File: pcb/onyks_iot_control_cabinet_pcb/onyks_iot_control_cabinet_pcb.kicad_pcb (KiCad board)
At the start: 2 copper layers, 80 x 90 mm, 41 parts, among them J1 Conn_01x02_Socket, J10 Conn_02x05_Odd_Even, J2 Conn_01x06_Socket, J3 Screw_Terminal_01x02, J4 Jack-DC, J5 Conn_01x03_Pin, J6 Conn_02x09_Odd_Even, J7 Screw_Terminal_01x02, J8 Conn_01x06_Pin, Q1 SQ4050EY-T1_GE3, Q2 SQ4050EY-T1_GE3, Q3 NPN, Q4 NPN, SW1 SW_Push, SW2 SW_Push, SW3 SW_Push, U1 ESP32-WROOM-32D, U2 LMR51430

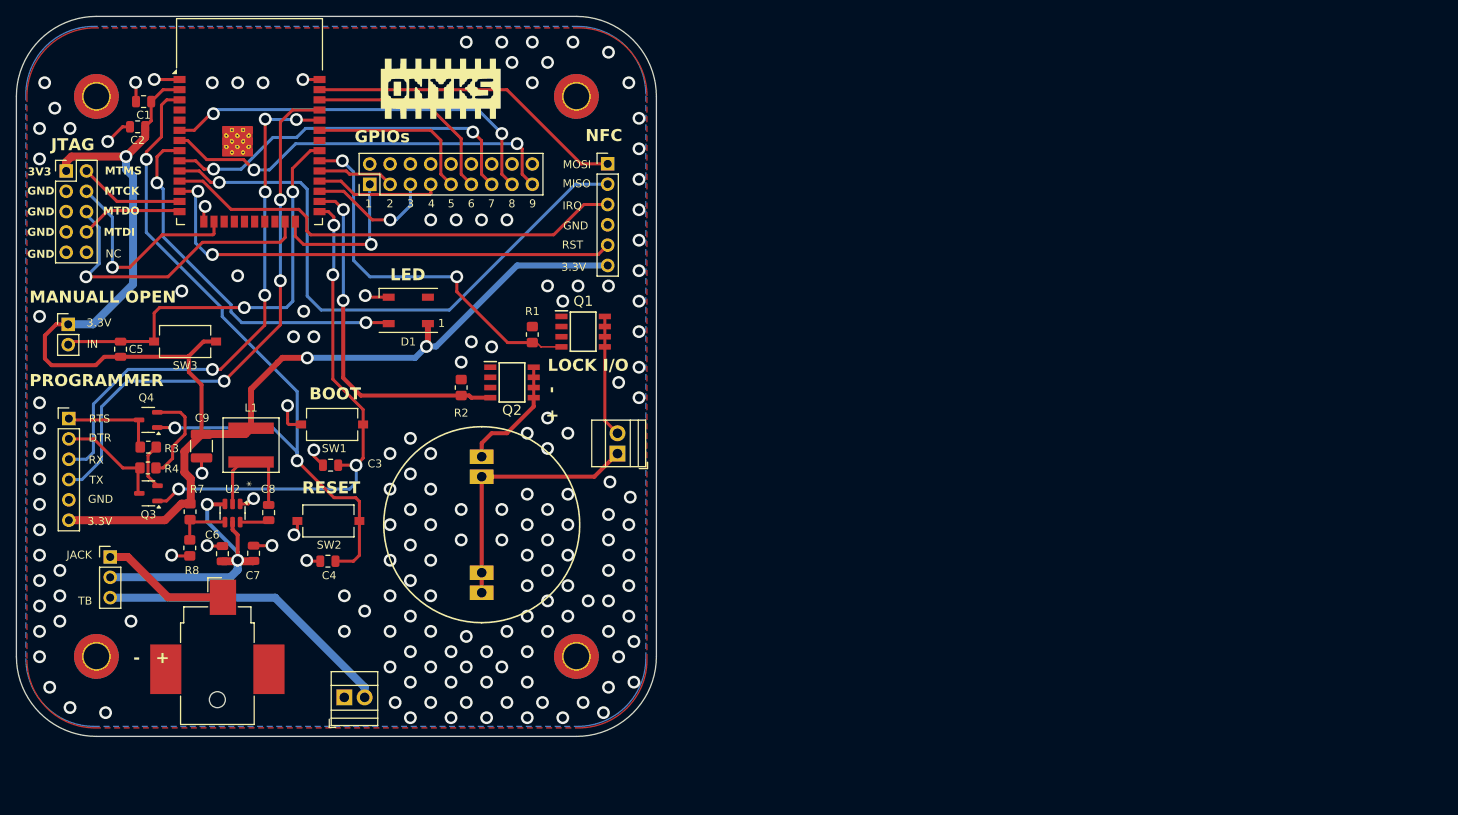
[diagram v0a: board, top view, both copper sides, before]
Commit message: PCB Overhaul
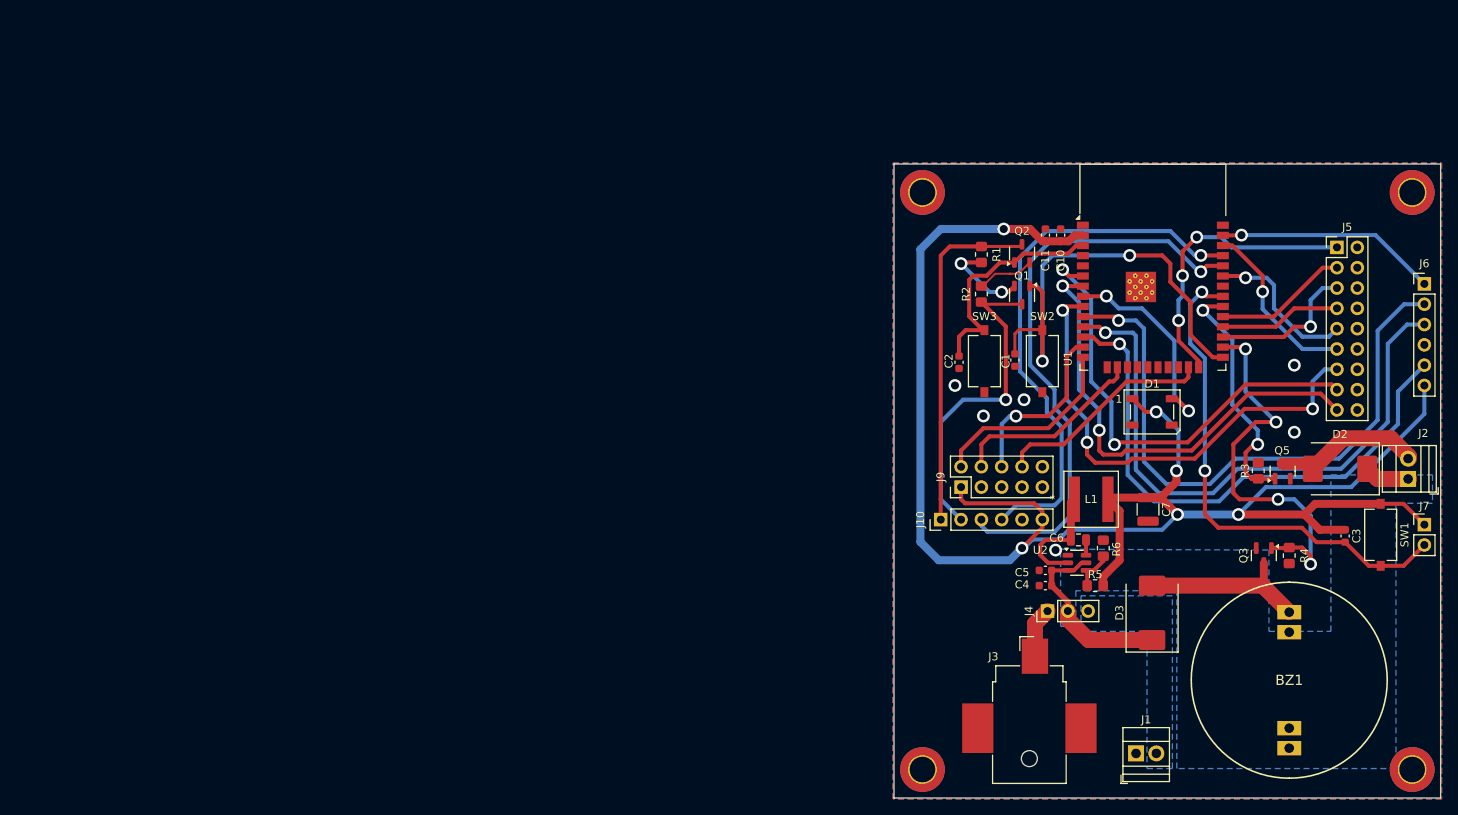
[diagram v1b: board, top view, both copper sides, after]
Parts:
- removed C8: 0.1u, Capacitor_SMD:C_0805_2012Metric
- removed C9: 100u, Capacitor_SMD:C_1210_3225Metric
- removed G***: LOGO, ourFootprints:LOGO
- removed J8: Conn_01x06_Pin, Connector_PinHeader_2.54mm:PinHeader_1x06_P2.54mm_Vertical
- removed Q4: NPN, Package_TO_SOT_SMD:SOT-23-3
- removed R7: 100k, Resistor_SMD:R_0805_2012Metric_Pad1.20x1.40mm_HandSolder
- removed R8: 22.1k, Resistor_SMD:R_0805_2012Metric_Pad1.20x1.40mm_HandSolder
- added C10: 22u/10V, Capacitor_SMD:C_0603_1608Metric, F.Cu at (176.5, 53.3)
- added C11: 0.1u/50V, Capacitor_SMD:C_0603_1608Metric, F.Cu at (174.6, 53.3)
- added D2: S5J, Diode_SMD:D_SMC, F.Cu at (211.5, 82.5)
- added D3: S5J, Diode_SMD:D_SMC, F.Cu at (188.0, 100.6)
- added J9: Conn_02x05_Odd_Even, Connector_PinHeader_2.54mm:PinHeader_2x05_P2.54mm_Vertical, F.Cu at (164.1, 84.8)
- added Q5: PMV100ENEAR, Package_TO_SOT_SMD:SOT-23, F.Cu at (204.3, 82.9)
- added R5: 100k, Resistor_SMD:R_0805_2012Metric_Pad1.20x1.40mm_HandSolder, F.Cu at (180.8, 97.2)
- added R6: 22.1k, Resistor_SMD:R_0805_2012Metric_Pad1.20x1.40mm_HandSolder, F.Cu at (181.9, 92.5)
- BZ1: value Buzzer -> CPI2416100T
- C1: value 22u -> 0.1u/50V; footprint Capacitor_SMD:C_0805_2012Metric -> Capacitor_SMD:C_0603_1608Metric
- C2, C3: value 0.1u -> 0.1u/50V; footprint Capacitor_SMD:C_0805_2012Metric -> Capacitor_SMD:C_0603_1608Metric
- C4: value 0.1u -> 2.2u/50V; footprint Capacitor_SMD:C_0805_2012Metric -> Capacitor_SMD:C_0603_1608Metric
- C5: value 0.1u -> 100n/50V; footprint Capacitor_SMD:C_0805_2012Metric -> Capacitor_SMD:C_0603_1608Metric
- C6: value 2.2u -> 100n/50V
- C7: value 100n -> 100u/6.3V; footprint Capacitor_SMD:C_0805_2012Metric -> Capacitor_SMD:C_1210_3225Metric
- J1: value Conn_01x02_Socket -> Screw_Terminal_01x02; footprint Connector_PinHeader_2.54mm:PinHeader_1x02_P2.54mm_Vertical -> TerminalBlock:TerminalBlock_Xinya_XY308-2.54-2P_1x02_P2.54mm_Horizontal
- J10: value Conn_02x05_Odd_Even -> Conn_01x06_Pin; footprint Connector_PinHeader_2.54mm:PinHeader_2x05_P2.54mm_Vertical -> Connector_PinHeader_2.54mm:PinHeader_1x06_P2.54mm_Vertical
- J2: value Conn_01x06_Socket -> Screw_Terminal_01x02; footprint Connector_PinHeader_2.54mm:PinHeader_1x06_P2.54mm_Vertical -> TerminalBlock:TerminalBlock_Xinya_XY308-2.54-2P_1x02_P2.54mm_Horizontal
- J3: value Screw_Terminal_01x02 -> Jack-DC; footprint TerminalBlock:TerminalBlock_Xinya_XY308-2.54-2P_1x02_P2.54mm_Horizontal -> Connector_BarrelJack:BarrelJack_CUI_PJ-036AH-SMT_Horizontal
- J4: value Jack-DC -> Conn_01x03_Pin; footprint Connector_BarrelJack:BarrelJack_CUI_PJ-036AH-SMT_Horizontal -> Connector_PinHeader_2.54mm:PinHeader_1x03_P2.54mm_Vertical
- J5: value Conn_01x03_Pin -> Conn_02x09_Odd_Even; footprint Connector_PinHeader_2.54mm:PinHeader_1x03_P2.54mm_Vertical -> Connector_PinHeader_2.54mm:PinHeader_2x09_P2.54mm_Vertical
- J6: value Conn_02x09_Odd_Even -> Conn_01x06_Socket; footprint Connector_PinHeader_2.54mm:PinHeader_2x09_P2.54mm_Vertical -> Connector_PinHeader_2.54mm:PinHeader_1x06_P2.54mm_Vertical
- J7: value Screw_Terminal_01x02 -> Conn_01x02_Socket; footprint TerminalBlock:TerminalBlock_Xinya_XY308-2.54-2P_1x02_P2.54mm_Horizontal -> Connector_PinHeader_2.54mm:PinHeader_1x02_P2.54mm_Vertical
- L1: value 5.6u -> XAL6060-562MEC_COC
- Q1, Q2: value SQ4050EY-T1_GE3 -> NPN; footprint ourFootprints:SOIC127P600X175-8N -> Package_TO_SOT_SMD:SOT-23-3
- Q3: value NPN -> PMV100ENEAR; footprint Package_TO_SOT_SMD:SOT-23-3 -> Package_TO_SOT_SMD:SOT-23
- R1, R2: value 100 -> 10k
- R3, R4: value 10k -> 100
- U2: value LMR51430 -> LMR51430XDDCR
- moved H3 184.7 mm to (220.5, 120.1)
- moved J5 158.2 mm to (211.1, 54.9)
- moved J1 143.8 mm to (186.0, 118.1)
- moved R4 143.1 mm to (205.1, 93.4), turned to -90 degrees
- moved Q3 139.6 mm to (201.9, 93.4), turned to -90 degrees
- moved R3 138.8 mm to (201.2, 82.8), turned to 90 degrees
- moved J6 132.4 mm to (222.0, 59.4), turned to 0 degrees
- moved SW1 131.8 mm to (216.5, 90.8), turned to -90 degrees
- moved C3 127.1 mm to (212.1, 90.9), turned to -90 degrees
- moved C5 118.9 mm to (174.6, 95.2), turned to 180 degrees
- moved J10 117.7 mm to (161.5, 88.9), turned to 90 degrees
- moved U1 114.4 mm to (188.1, 60.4)
- moved C1 113.6 mm to (170.8, 69.0), turned to -90 degrees
- moved C7 111.9 mm to (187.5, 87.6), turned to -90 degrees
- moved J2 107.5 mm to (220.0, 83.8), turned to 90 degrees
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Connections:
- net Net-(D1-DIN) renamed /MCU/GPIO_32
- BZ1 pad A1: LOCK_PLUS -> +12V
- BZ1 pad B1: LOCK_PLUS -> +12V
- BZ1 pad B2: LOCK_PLUS -> +12V
- C1 pad 1: +3.3V -> /MCU/MCU_BOOT
- C2 pad 1: +3.3V -> /MCU/MCU_RESET
- C3 pad 1: GND -> +3.3V
- C3 pad 2: MCU_BOOT -> /MCU/GPIO_19
- C4 pad 1: GND -> +12V
- C4 pad 2: MCU_RESET -> GND
- C5 pad 1: +3.3V -> +12V
- C5 pad 2: LOCK_MCU_MANUAL_OPEN -> GND
- C6 pad 1: V_IN -> Net-(U2-CB)
- C6 pad 2: GND -> Net-(U2-SW)
- C7 pad 1: V_IN -> +3.3V
- J1 pad 1: +3.3V -> GND
- J1 pad 2: LOCK_MCU_MANUAL_OPEN -> Net-(J1-Pin_2)
- J10 pad 1: +3.3V -> /MCU/RTS
- J10 pad 2: JTAG_MTMS -> /MCU/DTR
- J10 pad 3: GND -> /MCU/RXD
- J10 pad 4: JTAG_MTCK -> /MCU/TXD
- J10 pad 6: JTAG_MTDO -> +3.3V
- J2 pad 1: NFC_MOSI -> +12V
- J2 pad 2: NFC_MISO -> Net-(D2-A)
- J3 pad 1: GND -> Net-(J4-Pin_1)
- J3 pad 2: Net-(J3-Pin_2) -> GND
- J4 pad 1: Net-(J5-Pin_1) -> Net-(J4-Pin_1)
- J4 pad 2: GND -> +12V
- J4 pad 3: GND -> Net-(J1-Pin_2)
- J5 pad 1: Net-(J5-Pin_1) -> /MCU/GPIO_2
- J5 pad 2: V_IN -> GND
- J5 pad 3: Net-(J3-Pin_2) -> /MCU/GPIO_5
- J6 pad 1: FREE_GPIO_1 -> /MCU/GPIO_23
- J6 pad 2: GND -> /MCU/GPIO_25
- J6 pad 3: FREE_GPIO_2 -> /MCU/GPIO_26
- J6 pad 5: FREE_GPIO_3 -> /MCU/GPIO_27
- J6 pad 6: GND -> +3.3V
- J7 pad 1: LOCK_PLUS -> +3.3V
- J7 pad 2: LOCK_MINUS -> /MCU/GPIO_19
- Q1 pad 1: GND -> /MCU/MCU_BOOT
- Q1 pad 2: GND -> Net-(Q1-B)
- Q1 pad 3: GND -> /MCU/DTR
- Q2 pad 1: GND -> /MCU/MCU_RESET
- Q2 pad 2: GND -> Net-(Q2-B)
- Q2 pad 3: GND -> /MCU/RTS
- Q3 pad 1: MCU_BOOT -> /MCU/GPIO_4
- Q3 pad 2: Net-(Q3-B) -> GND
- Q3 pad 3: DTR -> Net-(BZ1--_2)
- R1 pad 1: LOCK_SWITCH -> Net-(Q1-B)
- R1 pad 2: GND -> /MCU/RTS
- R2 pad 1: BUZZER_SWITCH -> Net-(Q2-B)
- R2 pad 2: GND -> /MCU/DTR
- R3 pad 1: Net-(Q3-B) -> /MCU/GPIO_18
- R3 pad 2: RTS -> GND
- R4 pad 1: Net-(Q4-B) -> /MCU/GPIO_4
- R4 pad 2: DTR -> GND
- SW1 pad 1: GND -> +3.3V
- SW1 pad 2: MCU_BOOT -> /MCU/GPIO_19
- SW2 pad 1: GND -> /MCU/MCU_BOOT
- SW2 pad 2: MCU_RESET -> GND
- SW3 pad 1: +3.3V -> /MCU/MCU_RESET
- SW3 pad 2: LOCK_MCU_MANUAL_OPEN -> GND
- U1 pad 10: NFC_MISO -> /MCU/GPIO_25
- U1 pad 11: NFC_IRQ -> /MCU/GPIO_26
- U1 pad 12: NFC_RST -> /MCU/GPIO_27
- U1 pad 13: JTAG_MTMS -> /MCU/MTMS
- U1 pad 14: JTAG_MTDI -> /MCU/MTDI
- U1 pad 16: JTAG_MTCK -> /MCU/MTCK
- U1 pad 23: JTAG_MTDO -> /MCU/MTDO
- U1 pad 24: FREE_GPIO_1 -> /MCU/GPIO_2
- U1 pad 25: MCU_BOOT -> /MCU/MCU_BOOT
- U1 pad 26: BUZZER_SWITCH -> /MCU/GPIO_4
- U1 pad 27: FREE_GPIO_3 -> /MCU/GPIO_16
- U1 pad 28: FREE_GPIO_4 -> /MCU/GPIO_17
- U1 pad 29: FREE_GPIO_2 -> /MCU/GPIO_5
- U1 pad 3: MCU_RESET -> /MCU/MCU_RESET
- U1 pad 30: LOCK_SWITCH -> /MCU/GPIO_18
- U1 pad 31: LOCK_MCU_MANUAL_OPEN -> /MCU/GPIO_19
- U1 pad 33: FREE_GPIO_5 -> /MCU/GPIO_21
- U1 pad 34: MCU_RX_PROG -> /MCU/RXD
- U1 pad 35: MCU_TX_PROG -> /MCU/TXD
- U1 pad 36: FREE_GPIO_6 -> /MCU/GPIO_22
- U1 pad 37: NFC_MOSI -> /MCU/GPIO_23
- U1 pad 6: FREE_GPIO_8 -> /MCU/GPIO_34
- U1 pad 7: FREE_GPIO_9 -> /MCU/GPIO_35
- U1 pad 9: FREE_GPIO_7 -> /MCU/GPIO_33
- U2 pad 3: V_IN -> +12V
- U2 pad 5: V_IN -> +12V
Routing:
- net MCU_RESET: track 95.5 -> 0.00 mm, vias 3 -> 0
- net /MCU/GPIO_25: track 0.00 -> 77.0 mm, vias 0 -> 1
- net /MCU/GPIO_26: track 0.00 -> 75.6 mm, vias 0 -> 1
- net NFC_MISO: track 75.1 -> 0.00 mm, vias 1 -> 0
- net /MCU/RXD: track 0.00 -> 73.9 mm, vias 0 -> 1
- net /MCU/GPIO_27: track 0.00 -> 69.6 mm, vias 0 -> 1
- net MCU_TX_PROG: track 69.2 -> 0.00 mm, vias 3 -> 0
- net /MCU/TXD: track 0.00 -> 68.9 mm, vias 0 -> 1
- net MCU_RX_PROG: track 67.6 -> 0.00 mm, vias 5 -> 0
- net MCU_BOOT: track 65.3 -> 0.00 mm, vias 4 -> 0
- net /MCU/GPIO_19: track 0.00 -> 63.4 mm, vias 0 -> 2
- net NFC_RST: track 61.5 -> 0.00 mm, vias 2 -> 0
- net /MCU/MCU_BOOT: track 0.00 -> 60.6 mm, vias 0 -> 2
- net /MCU/GPIO_33: track 0.00 -> 60.5 mm, vias 0 -> 3
- net /MCU/GPIO_35: track 0.00 -> 58.9 mm, vias 0 -> 2
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- added copper zone on B.Cu, net +12V
- added copper zone on B.Cu, net Net-(J1-Pin_2)
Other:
- board size 80 x 90 mm -> 68.3 x 79.2 mm
- board text removed: "+"
- board text removed: "-"
- board text removed: "1"
- board text removed: "2"
- board text removed: "3"
- board text removed: "3.3V"
- board text removed: "3V3"
- board text removed: "4"
- board text removed: "5"
- board text removed: "6"
- board text removed: "7"
- board text removed: "8"
- board text removed: "9"
- board text removed: "BOOT"
- board text removed: "DTR"
- board text removed: "GND"
- board text removed: "GPIOs"
- board text removed: "IN"
- board text removed: "IRQ"
- board text removed: "JACK"
- board text removed: "JTAG"
- board text removed: "LED"
- board text removed: "LOCK I/O"
- board text removed: "MANUALL OPEN"
- board text removed: "MISO"
- board text removed: "MOSI"
- board text removed: "MTCK"
- board text removed: "MTDI"
- board text removed: "MTDO"
- board text removed: "MTMS"
- board text removed: "NC"
- board text removed: "NFC"
- board text removed: "PROGRAMMER"
- board text removed: "RESET"
- board text removed: "RST"
- board text removed: "RTS"
- board text removed: "RX"
- board text removed: "TB"
- board text removed: "TX"
